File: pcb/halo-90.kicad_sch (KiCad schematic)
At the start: 111 parts, among them U1 UFQFPN28, U2 LSM6DSM

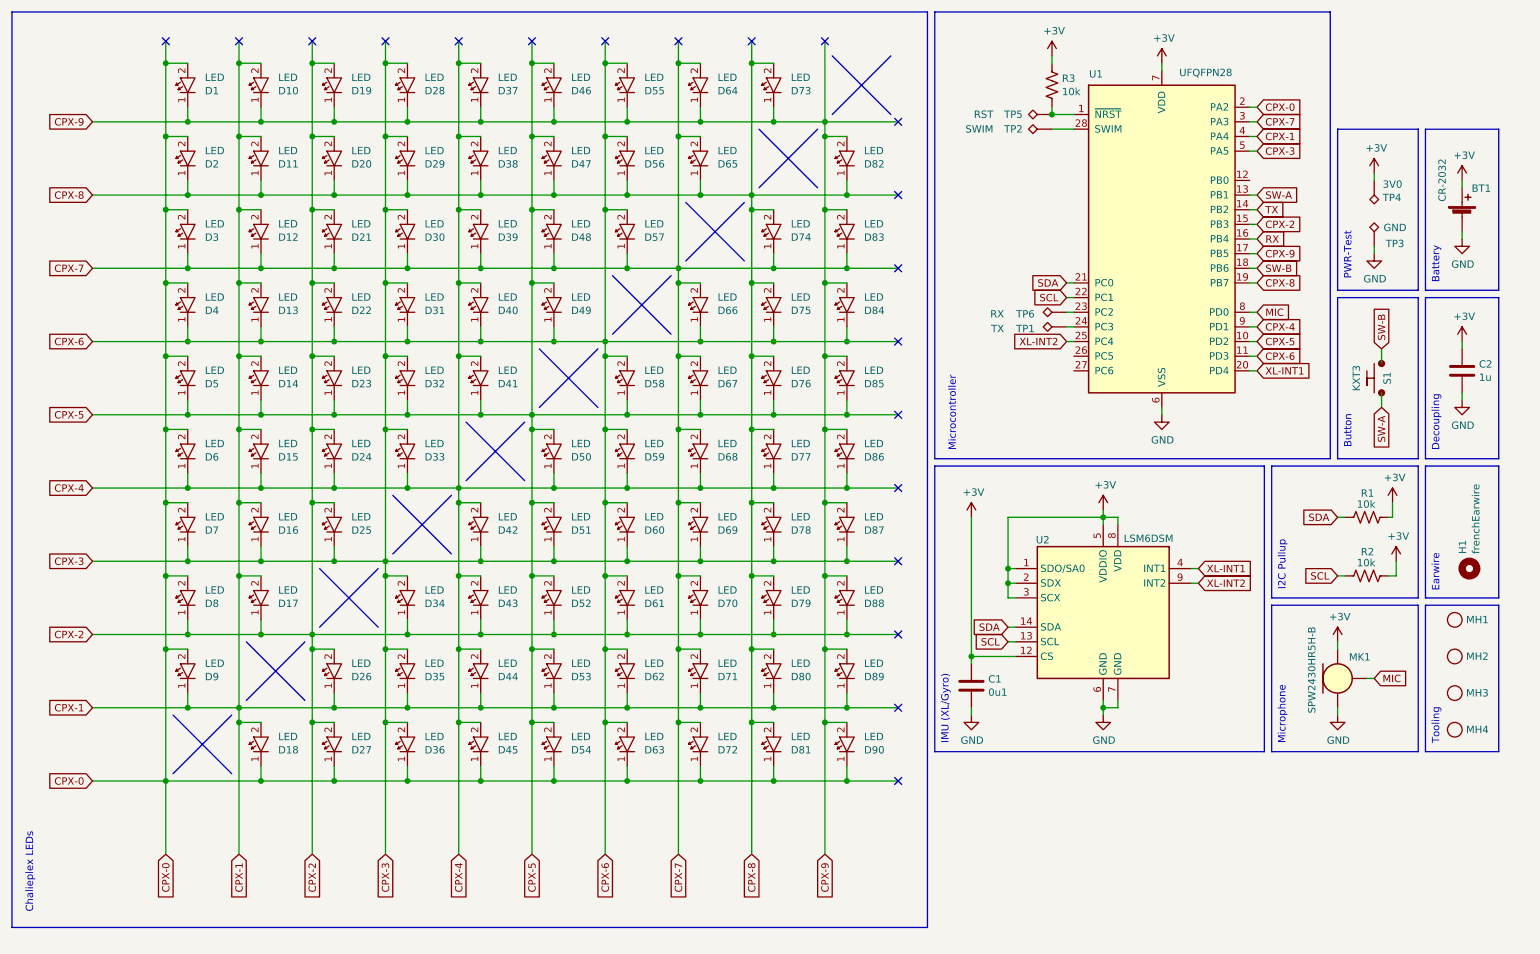
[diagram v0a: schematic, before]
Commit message: Acceleometer shcematic done?
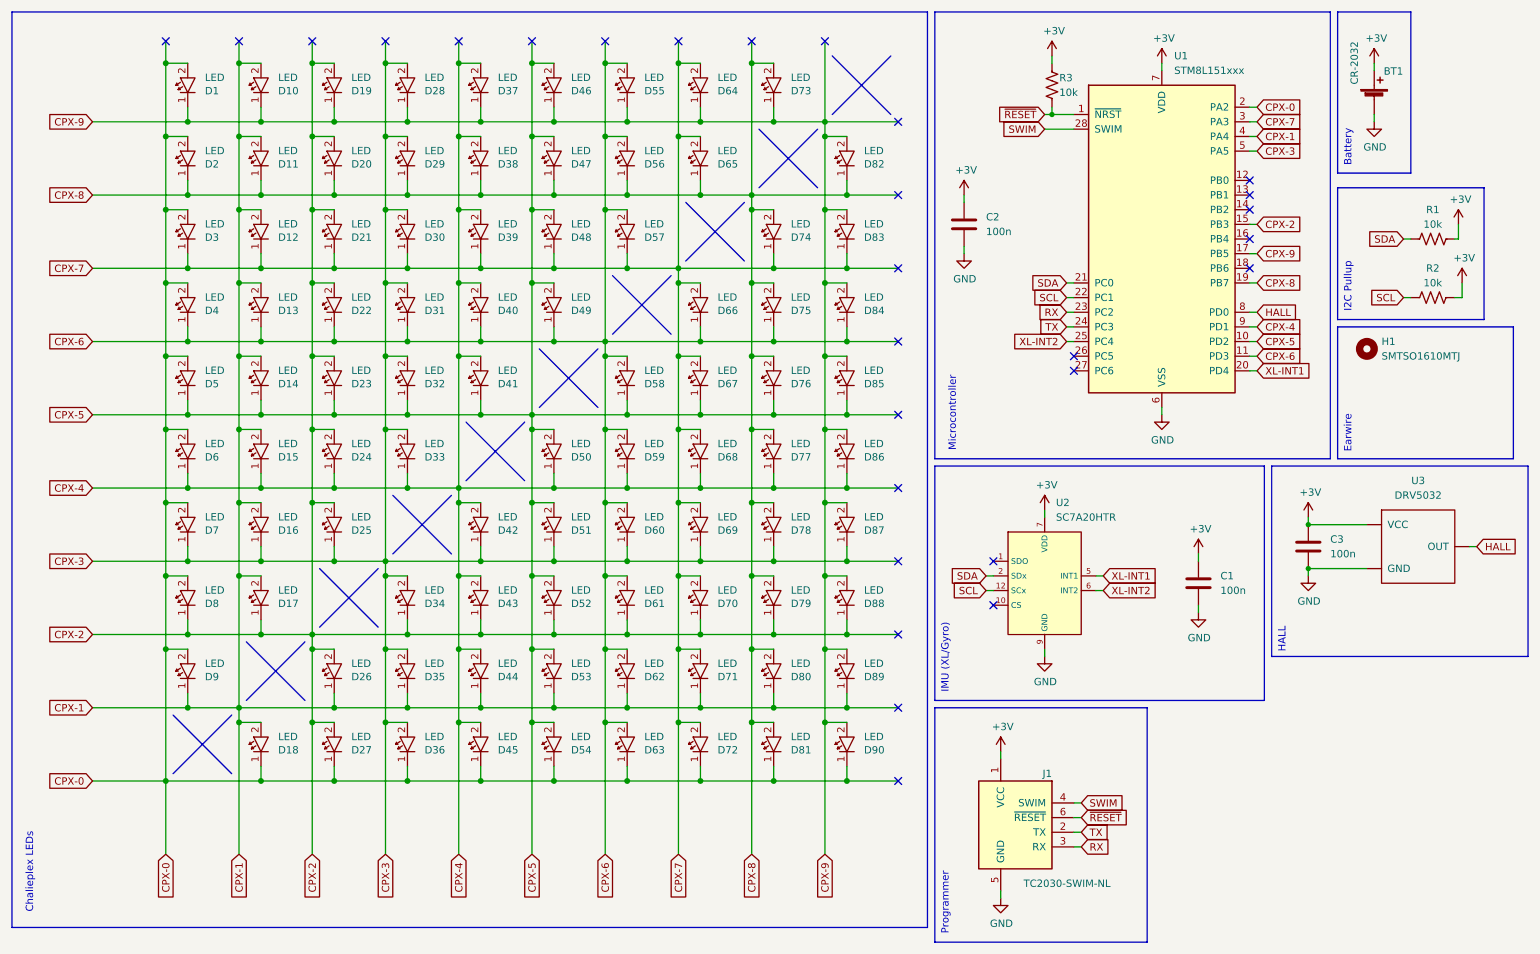
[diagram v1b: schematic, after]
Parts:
- removed C1: 0u1, passives:C-0402, symbol passives:C-0402
- removed C2: 1u, passives:C-0402, symbol passives:C-0402
- removed H1: frenchEarwire, frenchEarwire:frenchEarwire, symbol frenchEarwire:frenchEarwire
- removed MH1, MH2, MH3, MH4: toolingHole, tooling:1.152mm-ToolingHole, symbol tooling:toolingHole
- removed MK1: SPW2430HR5H-B, SPW2430HR5H-B:SPW2430HR5H-B, symbol SPW2430HR5H-B:SPW2430HR5H-B
- removed R1, R2, R3: 10k, passives:R-0402, symbol passives:R-0402
- removed S1: KXT3, KXT3:KXT3, symbol KXT3:KXT3
- removed TP1: TX, tooling:TestPoint_Pad_D1.0mm, symbol tooling:TestPoint_D1.0
- removed TP2: SWIM, tooling:TestPoint_Pad_D1.0mm, symbol tooling:TestPoint_D1.0
- removed TP3: GND, tooling:TestPoint_Pad_D1.0mm, symbol tooling:TestPoint_D1.0
- removed TP4: 3V0, tooling:TestPoint_Pad_D1.0mm, symbol tooling:TestPoint_D1.0
- removed TP5: RST, tooling:TestPoint_Pad_D1.0mm, symbol tooling:TestPoint_D1.0
- removed TP6: RX, tooling:TestPoint_Pad_D1.0mm, symbol tooling:TestPoint_D1.0
- removed U1: UFQFPN28, STM8L15xxx:UFQFPN28, symbol STM8L15xxx:UFQFPN28
- removed U2: LSM6DSM, LSM6DSM:LGA-14_3x2.5mm_6-6, symbol LSM6DSM:LSM6DSM
- added C1, C2, C3: 100n, C-0402:C-0402, symbol C-0402:100n
- added H1: SMTSO1610MTJ, SMTSO1610MTJ:SMTSO1610MTJ, symbol SMTSO1610MTJ:SMTSO1610MTJ
- added J1: TC2030-SWIM-NL, TC2030-IDC-NL:Tag-Connect_TC2030-IDC-NL_2x03_P1.27mm_Vertical, symbol TC2030-IDC-NL:TC2030-SWIM-NL
- added R1, R2, R3: 10k, R-0402:R-0402, symbol R-0402:10k
- added U1: STM8L151xxx, STM8L15xxx:UFQFPN28, symbol STM8L15xxx:STM8L151xxx
- added U2: SC7A20HTR, SC7A20HTR:SC7A20HTR, symbol SC7A20HTR:SC7A20HTR
- added U3: DRV5032, DRV5032:DRV5032, symbol DRV5032:DRV5032
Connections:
- net +3V: now also C1.1, C2.1, C3.1, J1.1 (VCC), R1.2, R2.2, R3.1, U1.7 (VDD), U2.3 (VDDIO), U2.7 (VDD), U3.1 (VCC)
- net CPX-0: now also U1.2 (PA2)
- net CPX-1: now also U1.4 (PA4)
- net CPX-2: now also U1.15 (PB3)
- net CPX-3: now also U1.5 (PA5)
- net CPX-4: now also U1.9 (PD1)
- net CPX-5: now also U1.10 (PD2)
- net CPX-6: now also U1.11 (PD3)
- net CPX-7: now also U1.3 (PA3)
- net CPX-8: now also U1.19 (PB7)
- net CPX-9: now also U1.17 (PB5)
- net GND: now also C1.2, C2.2, C3.2, J1.5 (GND), U1.6 (VSS), U2.8 (GNDIO), U2.9 (GND), U3.3 (GND)
- net RX: now also J1.3 (RX), U1.23 (PC2)
- net SCL: now also R2.1, U1.22 (PC1), U2.12 (SCx)
- net SDA: now also R1.1, U1.21 (PC0), U2.2 (SDx)
- net TX: now also J1.2 (TX), U1.24 (PC3)
- net XL-INT1: now also U1.20 (PD4), U2.5 (INT1)
- net XL-INT2: now also U1.25 (PC4), U2.6 (INT2)
- new net HALL: U1.8 (PD0), U3.2 (OUT)
- new net SWIM: J1.4 (SWIM), U1.28 (SWIM)
- new net ~{RESET}: J1.6 (~{RESET}), R3.2, U1.1 (~{NRST})
- no-connect marks 20 -> 29
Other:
- note added: "HALL"
- note added: "Programmer"
- note removed: "Button"
- note removed: "Decoupling"
- note removed: "Microphone"
- note removed: "PWR-Test"
- note removed: "Tooling"
- moved on the sheet: BT1
